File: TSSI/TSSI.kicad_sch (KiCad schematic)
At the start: 134 parts, among them J1 Conn_01x04_Pin, J2 Conn_01x02_Pin, J3 Conn_01x03_Pin, J4 Conn_01x02_Pin, U2 M74VHC1GT32DFT1G, U3 LM555xN, U4 SN74AHC1G02MDCKREP, U5 LD1086DT50TR

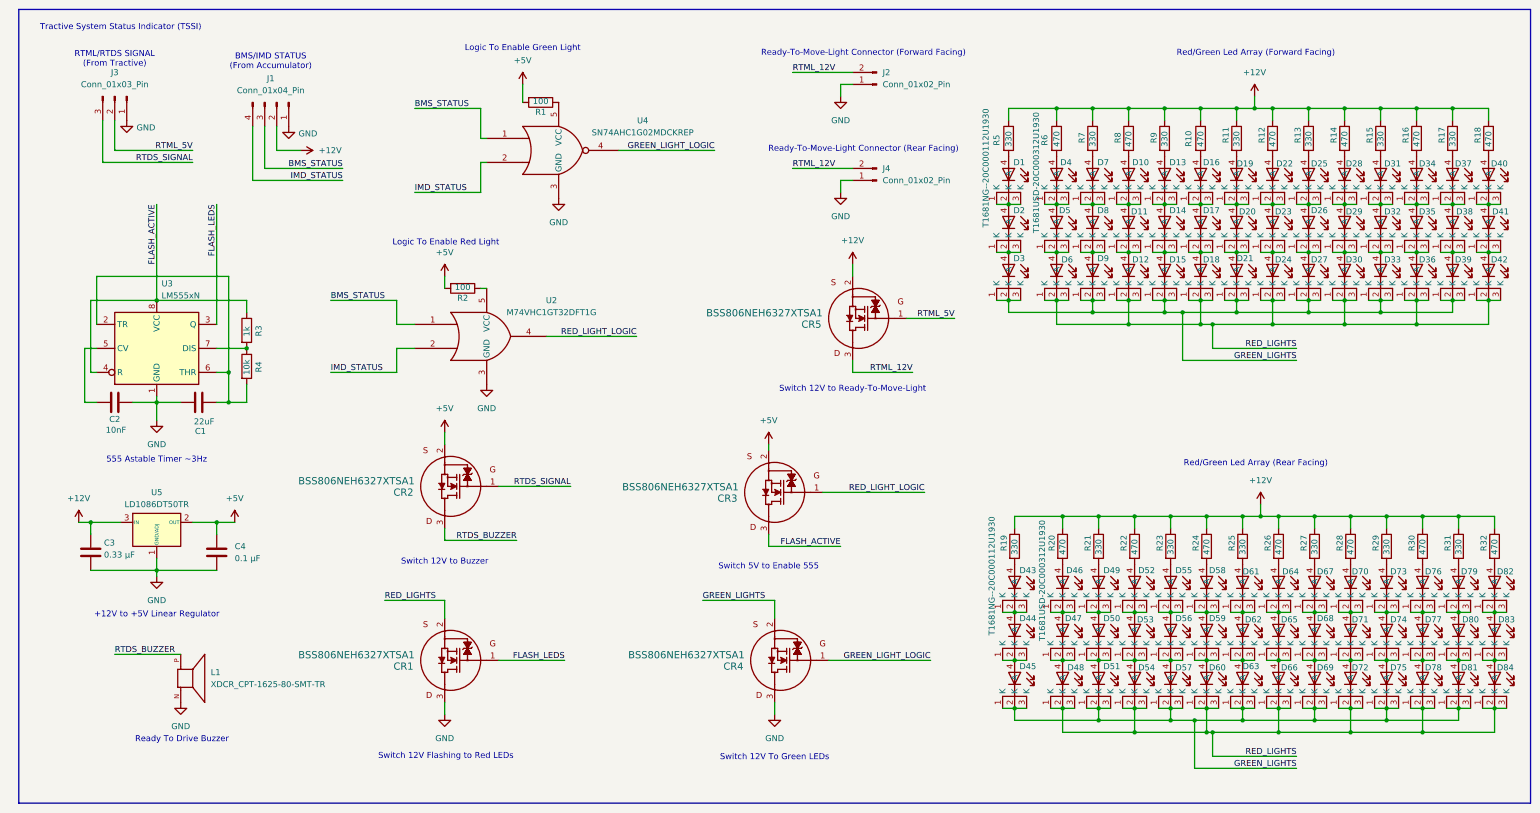
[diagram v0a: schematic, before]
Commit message: TSSI_v2.0 Final Commit
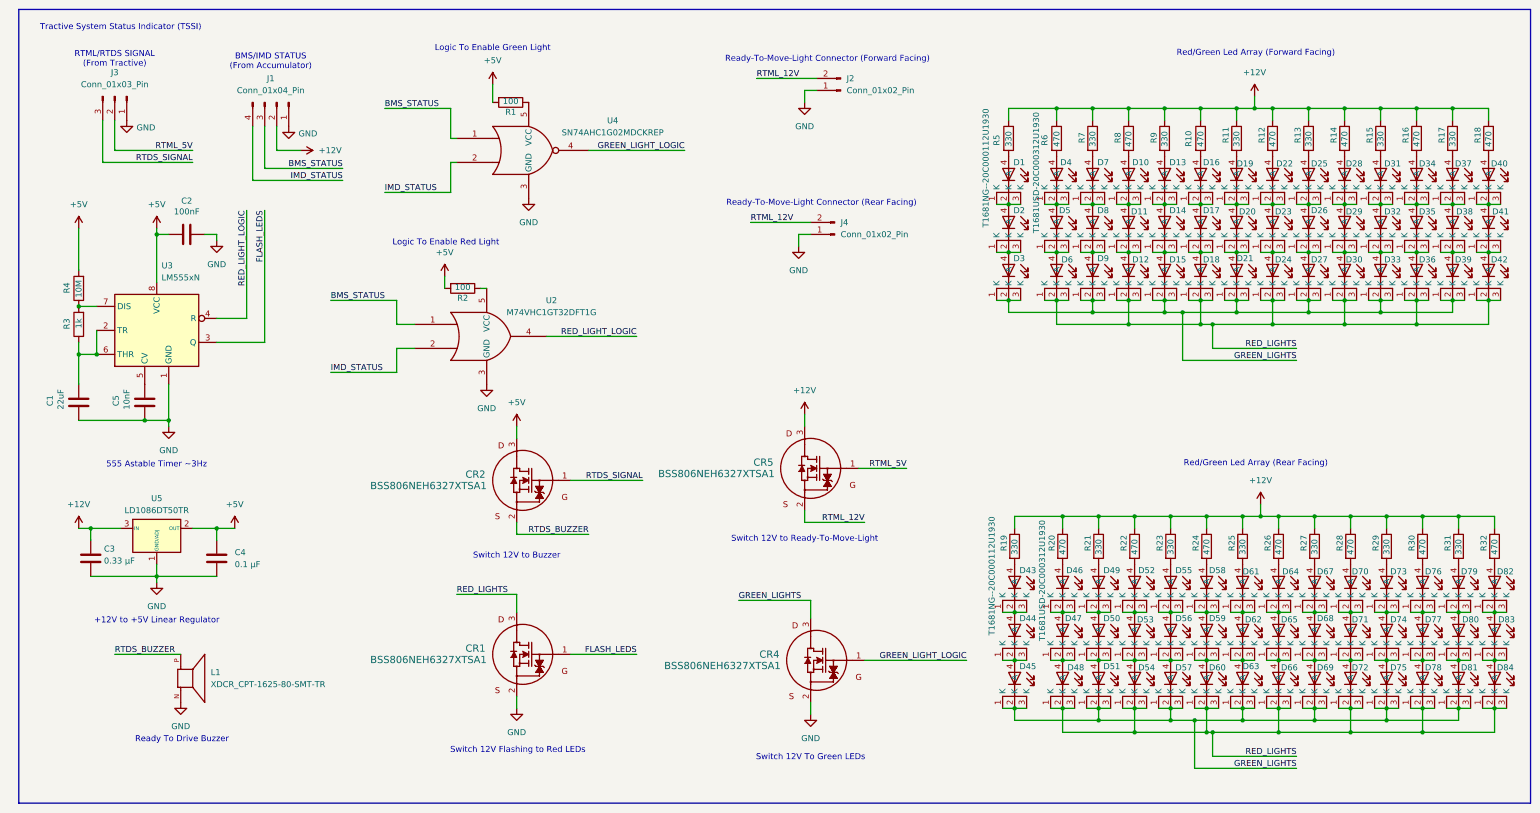
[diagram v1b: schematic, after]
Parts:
- removed CR3: BSS806NEH6327XTSA1, Footprints:PG-SOT23-3-5_INF, symbol 2025-02-02_06-48-36:BSS806NEH6327XTSA1
- added C5: 10nF, Capacitor_SMD:C_0805_2012Metric_Pad1.18x1.45mm_HandSolder, symbol Device:C
- C2: value 10nF -> 100nF
- R4: value 10k -> 10M
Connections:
- net +12V: now also CR5.3; no longer CR5.2
- net +5V: now also C2.1, CR2.3, R4.2, U3.8 (VCC); no longer CR2.2
- net GND: now also CR1.2, CR4.2, C5.1; no longer CR1.3, CR4.3
- net GREEN_LIGHTS: now also CR4.3; no longer CR4.2
- net RED_LIGHTS: now also CR1.3; no longer CR1.2
- net RED_LIGHT_LOGIC: now also U3.4 (R)
- net RTDS_BUZZER: now also CR2.2; no longer CR2.3
- net RTML_12V: now also CR5.2; no longer CR5.3
- net at C1.2, U3.2 (TR), U3.6 (THR): now also R3.1; no longer R4.2
- net at U3.5 (CV): now also C5.2; no longer C2.1
- removed net FLASH_ACTIVE: R3.1, U3.4 (R), U3.8 (VCC)
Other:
- note removed: "Switch 5V to Enable 555"
- moved on the sheet: C1, C2, C3, C4, CR1, CR2, CR4, CR5, J2, J4, R1, R3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
